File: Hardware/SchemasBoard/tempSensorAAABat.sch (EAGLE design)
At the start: 9 parts, among them IC1 DS1820

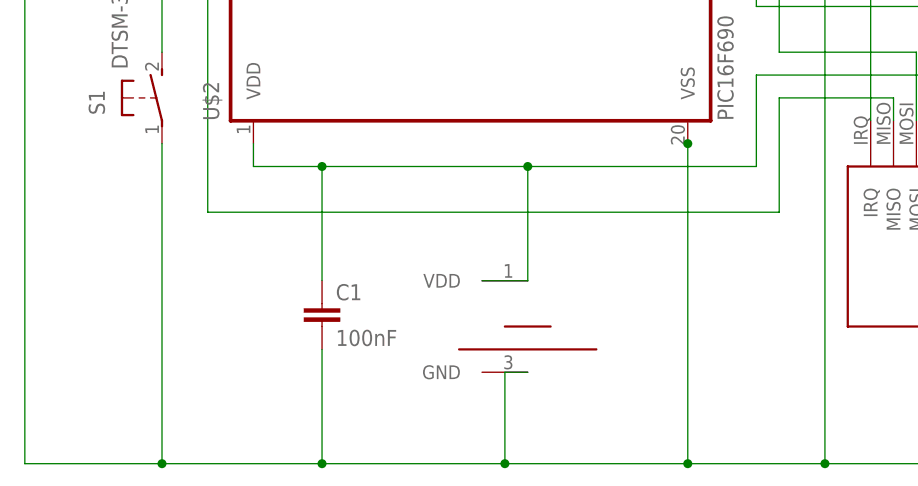
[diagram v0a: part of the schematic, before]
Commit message: aaa
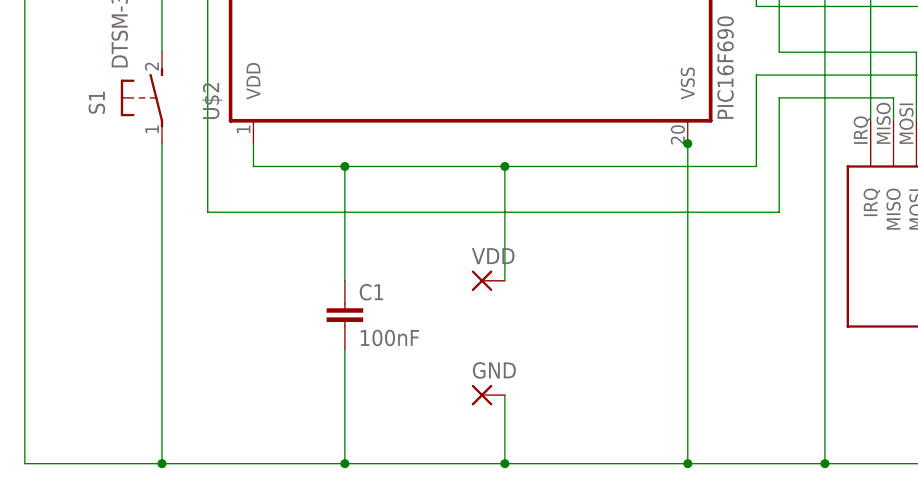
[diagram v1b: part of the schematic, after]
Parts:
- removed U$4: CR2032, rfm70:CR2032
- added GND, VDD: (no value), wirepad:SMD5
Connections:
- net N$5: now also VDD.P; no longer U$4.VDD
- net VD: now also GND.P; no longer U$4.GND
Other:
- moved on the sheet: C1
